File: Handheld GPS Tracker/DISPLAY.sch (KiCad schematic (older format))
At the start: 1 part

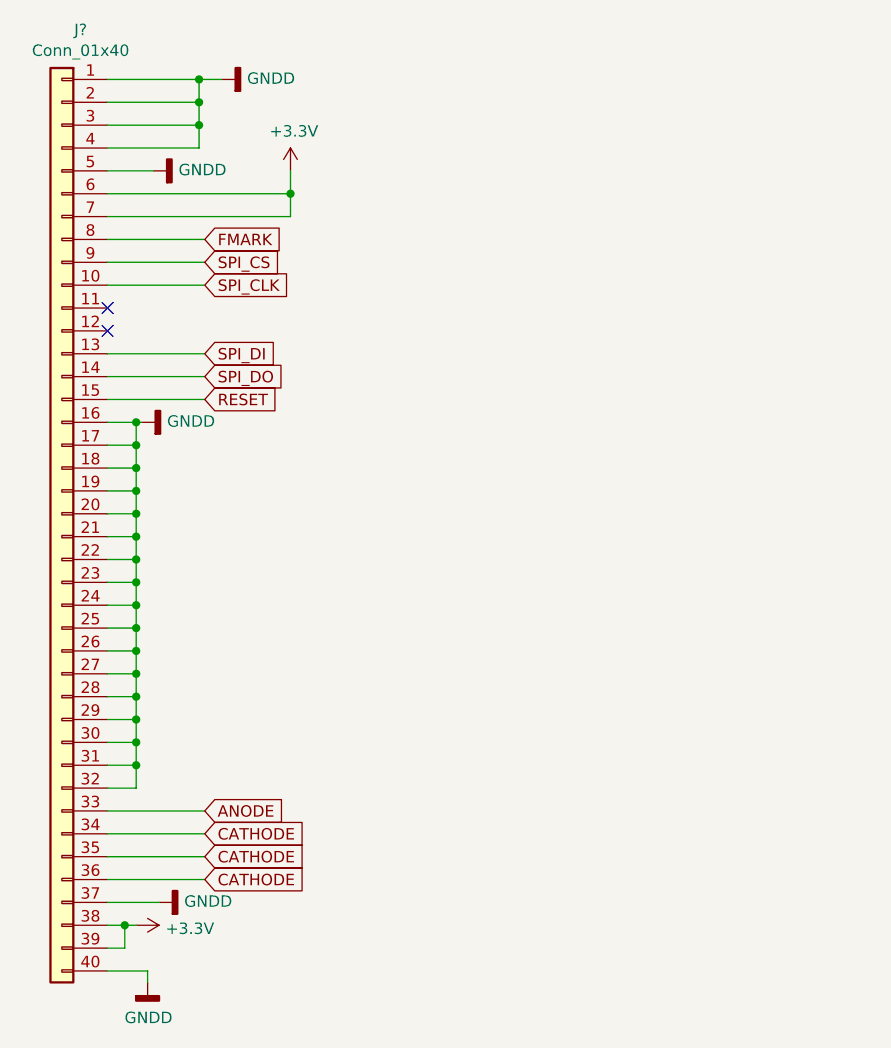
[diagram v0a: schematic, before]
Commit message: Add files via upload
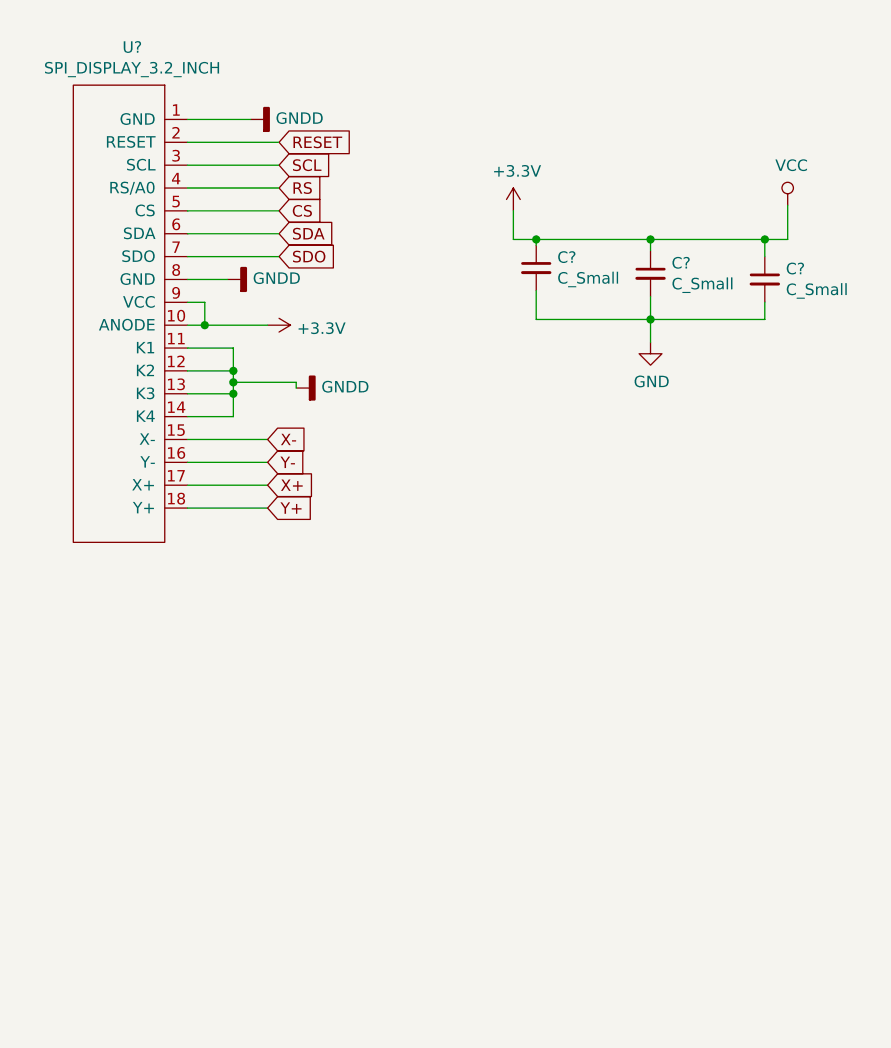
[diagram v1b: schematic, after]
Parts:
- removed J?: Conn_01x40, symbol Connector_Generic:Conn_01x40
- added C? (x3): C_Small, symbol Device:C_Small
- added U?: SPI_DISPLAY_3.2_INCH, ASSETS:ILI9341 TFT DISPLAY SPI, symbol ILI9341_SPI_DISPLAY:SPI_DISPLAY_3.2_INCH
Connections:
- net +3V3: now also C?.1, C?.1, C?.1, U?.10 (ANODE), U?.9 (VCC)
- net GNDD: now also U?.1 (GND), U?.11 (K1), U?.12 (K2), U?.13 (K3), U?.14 (K4), U?.8 (GND)
- net RESET: now also U?.2 (RESET)
- new net CS: U?.5 (CS)
- new net GND: C?.2, C?.2, C?.2
- new net RS: U?.4 (RS/A0)
- new net SCL: U?.3 (SCL)
- new net SDA: U?.6 (SDA)
- new net SDO: U?.7 (SDO)
- new net X+: U?.17 (X+)
- new net X-: U?.15 (X-)
- new net Y+: U?.18 (Y+)
- new net Y-: U?.16 (Y-)
- no-connect marks 2 -> 0

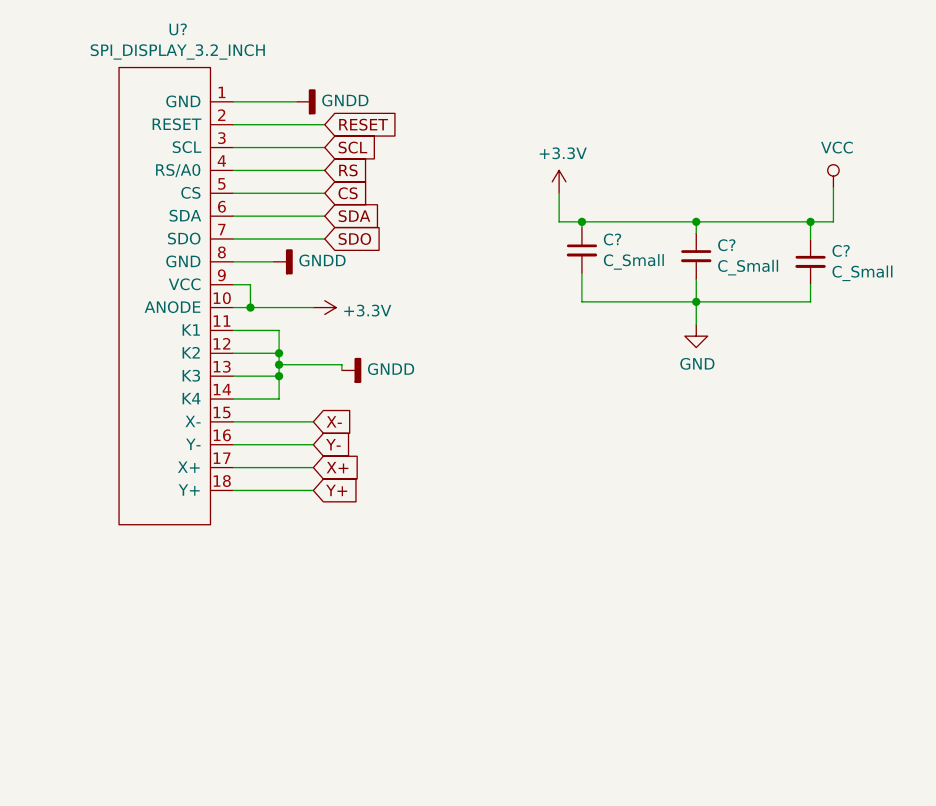
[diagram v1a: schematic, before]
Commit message: Add files via upload
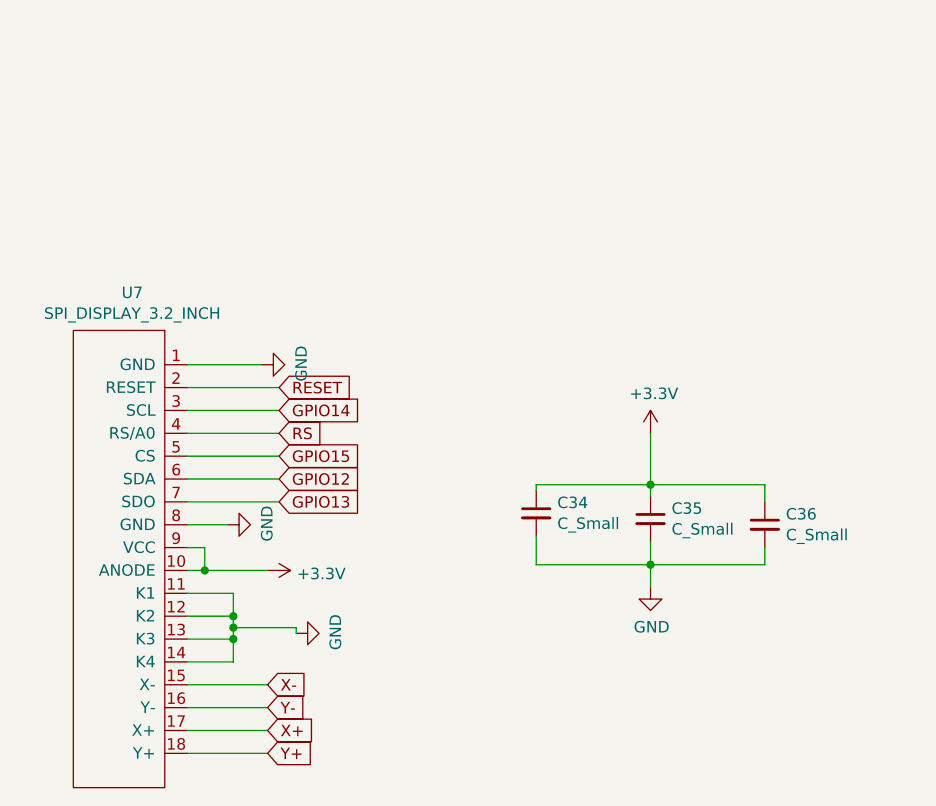
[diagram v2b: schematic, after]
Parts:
- gave numbers to parts that had none: 4
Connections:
- net GNDD is gone; now on net GND: U7.1 (GND), U7.11 (K1), U7.12 (K2), U7.13 (K3), U7.14 (K4), U7.8 (GND)
- net CS renamed GPIO15
- net SCL renamed GPIO14
- net SDA renamed GPIO12
- net SDO renamed GPIO13
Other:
- moved on the sheet: C34, C35, C36, U7

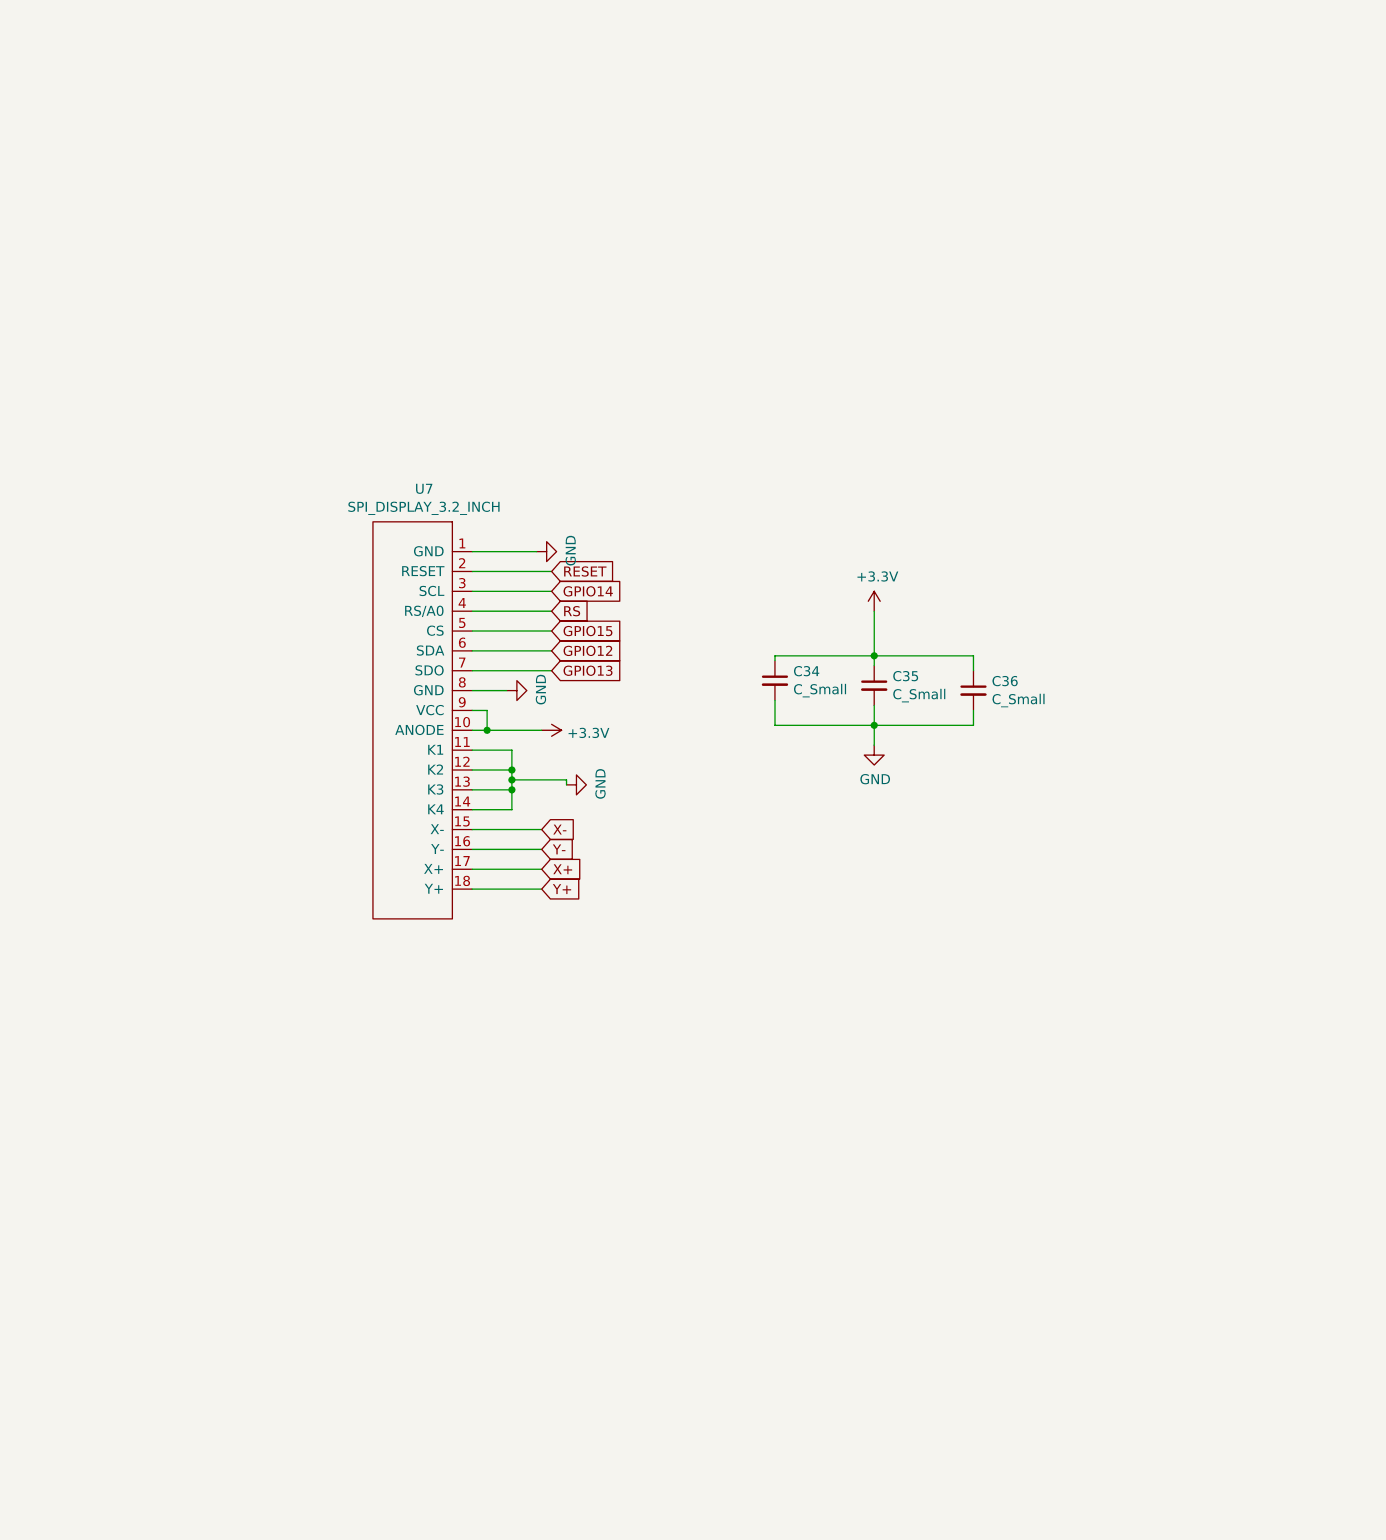
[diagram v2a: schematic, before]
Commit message: Add files via upload
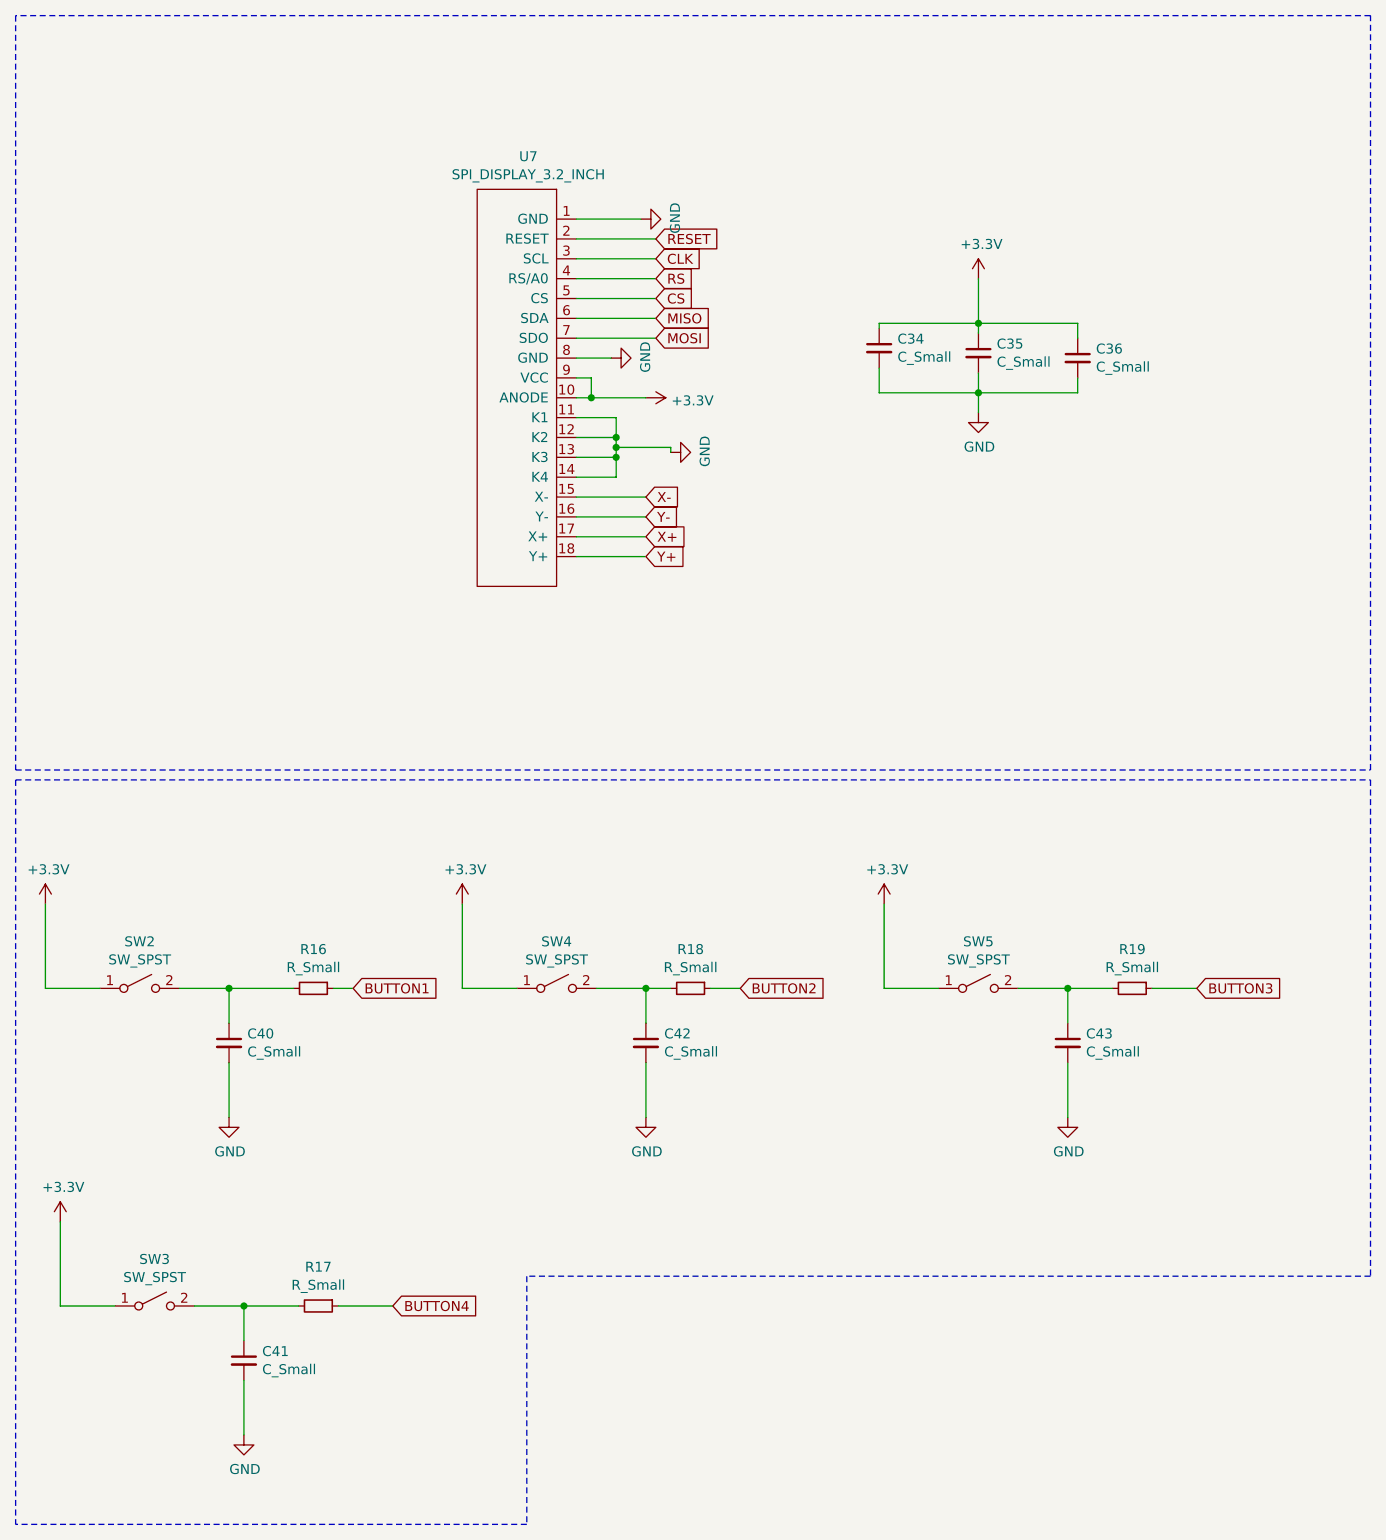
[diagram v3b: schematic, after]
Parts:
- added C40, C41, C42, C43: C_Small, Capacitor_SMD:C_0603_1608Metric, symbol Device:C_Small
- added R16, R17, R18, R19: R_Small, Resistor_SMD:R_0402_1005Metric, symbol Device:R_Small
- added SW2, SW3, SW4, SW5: SW_SPST, Button_Switch_THT:SW_PUSH_6mm_H8mm, symbol Switch:SW_SPST
- C34, C35, C36: footprint (none) -> Capacitor_SMD:C_0603_1608Metric
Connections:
- net +3V3: now also SW2.1 (A), SW3.1 (A), SW4.1 (A), SW5.1 (A)
- net GND: now also C40.2, C41.2, C42.2, C43.2
- net GPIO12 renamed MISO
- net GPIO13 renamed MOSI
- net GPIO14 renamed CLK
- net GPIO15 renamed CS
- new net: C40.1, R16.2, SW2.2 (B)
- new net: C42.1, R18.2, SW4.2 (B)
- new net: C43.1, R19.2, SW5.2 (B)
- new net: C41.1, R17.2, SW3.2 (B)
- new net BUTTON1: R16.1
- new net BUTTON2: R18.1
- new net BUTTON3: R19.1
- new net BUTTON4: R17.1
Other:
- moved on the sheet: C34, C35, C36, U7
